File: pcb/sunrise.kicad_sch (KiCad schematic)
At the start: 11 parts, among them J1 Conn_01x15_Female, J2 Conn_01x15_Female, J3 Conn_01x04_Female, J4 Conn_01x02_Female, Q1 TSM2302CX, Q2 TSM2302CX, Q3 TSM2302CX, U1 MCP1703A-5002_SOT223

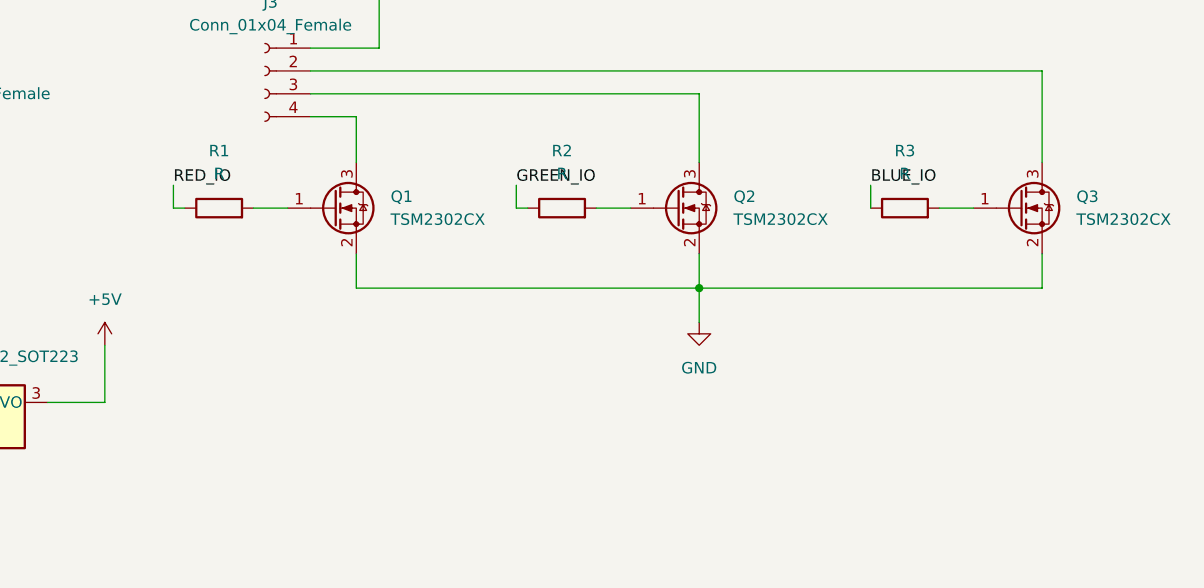
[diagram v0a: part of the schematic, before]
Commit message: Added resistor
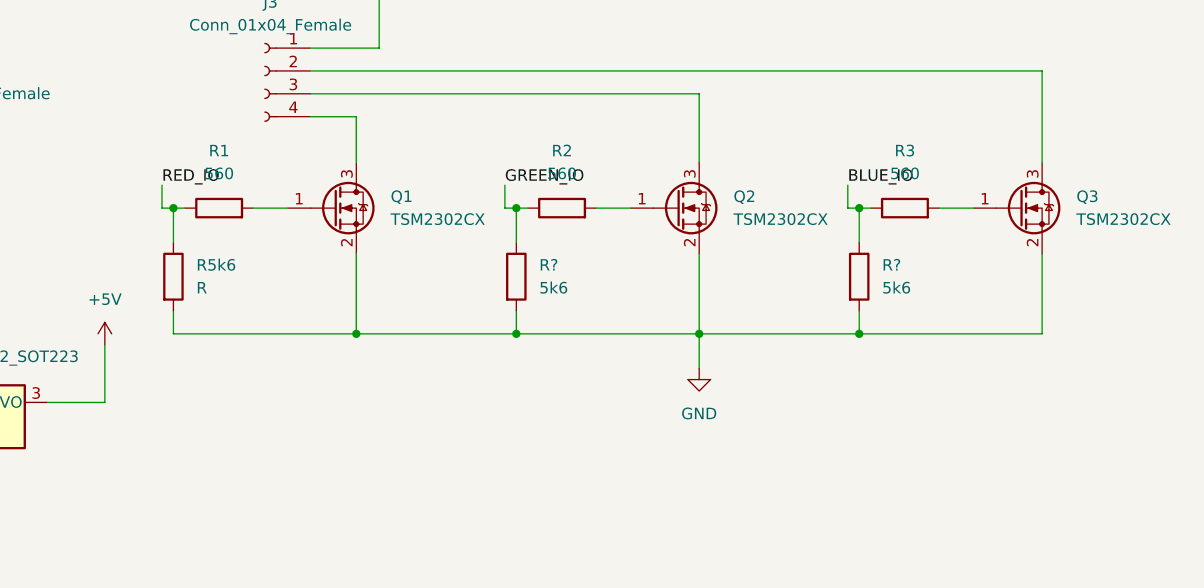
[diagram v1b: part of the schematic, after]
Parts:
- added R5k6: R, Resistor_SMD:R_0805_2012Metric, symbol Device:R
- added R? (x2): 5k6, Resistor_SMD:R_0805_2012Metric, symbol Device:R
- R1, R2, R3: value R -> 560
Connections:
- net BLUE_IO: now also R?.1
- net GND: now also R5k6.2, R?.2, R?.2
- net GREEN_IO: now also R?.1
- net RED_IO: now also R5k6.1
